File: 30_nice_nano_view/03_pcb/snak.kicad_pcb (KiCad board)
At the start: 2 copper layers, 114 x 99 mm, 162 parts

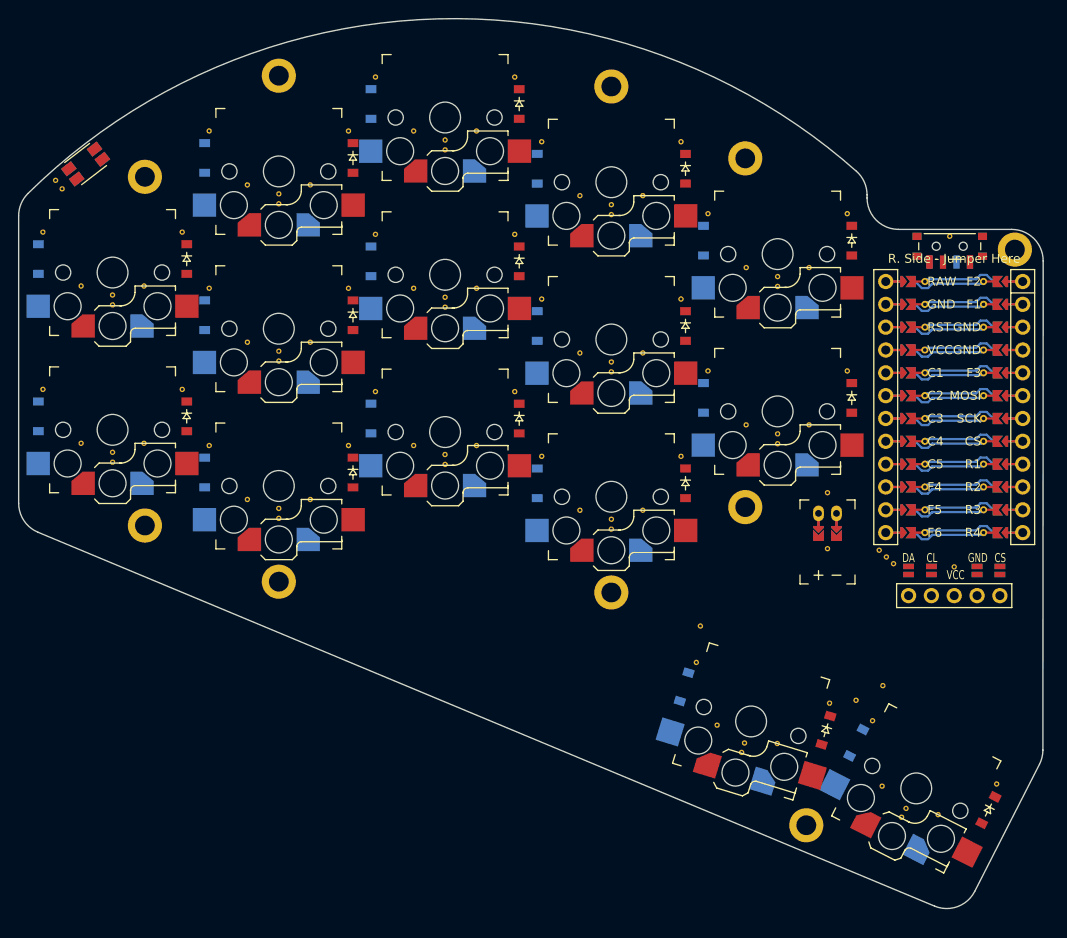
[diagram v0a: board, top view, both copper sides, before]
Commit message: update
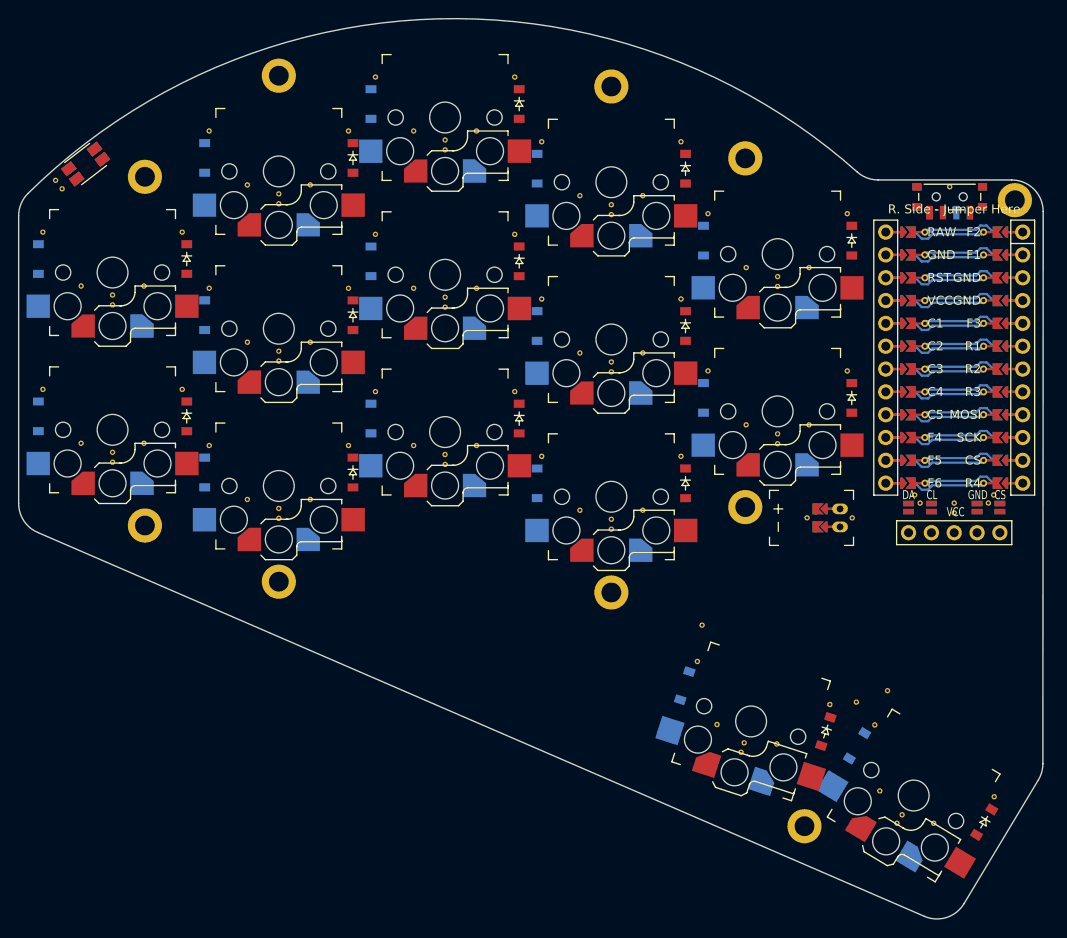
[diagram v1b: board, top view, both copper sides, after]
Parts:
- removed the REF** at (179.6, 89.5)
- removed the REF** at (179.8, 112.9)
- removed the REF** at (198.4, 121.9)
- removed the REF** at (174.0, 117.4)
- removed the REF** at (191.9, 125.3)
- removed the REF** at (165.0, 108.4)
- removed the REF** at (184.6, 114.9)
- removed the REF** at (167.3, 115.4)
- removed the REF** at (185.6, 122.1)
- removed the REF** at (170.0, 118.4)
- removed the REF** at (187.8, 125.6)
- removed the REF** at (170.3, 117.3)
- removed the REF** at (188.3, 124.6)
- removed the REF** at (182.7, 112.6)
- removed the REF** at (165.4, 104.3)
- removed the REF** at (185.7, 111.0)
- removed the REF** at (186.9, 97.4)
- removed the REF** at (186.1, 96.7)
- removed the REF** at (185.3, 95.9)
- removed the REF** at (193.7, 97.8)
- removed the REF** at (193.2, 61.0)
- removed the REF** at (179.6, 95.7)
- added REF**: VIA-0.6mm, VIA-0.6mm, F.Cu at (193.2, 55.5)
- added REF**: VIA-0.6mm, VIA-0.6mm, F.Cu at (177.3, 92.3)
- added REF**: VIA-0.6mm, VIA-0.6mm, F.Cu at (182.3, 92.3)
- added REF**: VIA-0.6mm, VIA-0.6mm, F.Cu at (179.8, 113.1)
- added REF**: VIA-0.6mm, VIA-0.6mm, F.Cu at (198.1, 123.3)
- added REF**: VIA-0.6mm, VIA-0.6mm, F.Cu at (173.9, 117.5)
- added REF**: VIA-0.6mm, VIA-0.6mm, F.Cu at (191.4, 126.3)
- added REF**: VIA-0.6mm, VIA-0.6mm, F.Cu at (165.1, 108.3)
- added REF**: VIA-0.6mm, VIA-0.6mm, F.Cu at (184.8, 115.3)
- added REF**: VIA-0.6mm, VIA-0.6mm, F.Cu at (167.3, 115.3)
- added REF**: VIA-0.6mm, VIA-0.6mm, F.Cu at (185.4, 122.7)
- added REF**: VIA-0.6mm, VIA-0.6mm, F.Cu at (169.9, 118.4)
- added REF**: VIA-0.6mm, VIA-0.6mm, F.Cu at (187.3, 126.3)
- added REF**: VIA-0.6mm, VIA-0.6mm, F.Cu at (170.3, 117.3)
- added REF**: VIA-0.6mm, VIA-0.6mm, F.Cu at (187.9, 125.3)
- added REF**: VIA-0.6mm, VIA-0.6mm, F.Cu at (182.8, 112.8)
- added REF**: VIA-0.6mm, VIA-0.6mm, F.Cu at (165.6, 104.2)
- added REF**: VIA-0.6mm, VIA-0.6mm, F.Cu at (186.2, 111.5)
- added REF**: VIA-0.6mm, VIA-0.6mm, F.Cu at (189.2, 89.8)
- added REF**: VIA-0.6mm, VIA-0.6mm, F.Cu at (198.1, 89.8)
- added REF**: VIA-0.6mm, VIA-0.6mm, F.Cu at (193.7, 90.7)
- added REF**: VIA-0.6mm, VIA-0.6mm, F.Cu at (189.8, 90.7)
- added REF**: VIA-0.6mm, VIA-0.6mm, F.Cu at (197.5, 90.7)
- added REF**: VIA-0.6mm, VIA-0.6mm, F.Cu at (193.7, 91.8)
- moved DISP1 7.00 mm to (193.7, 77.2)
- moved H10 5.50 mm to (200.4, 57.0)
- moved MCU1 5.50 mm to (193.7, 73.2)
- moved SW1 5.50 mm to (193.2, 56.6)
- moved JST1 1.49 mm to (180.9, 92.3), turned to 270 degrees
- moved D15 1.43 mm to (197.0, 126.2), turned to 239 degrees
- moved S15 0.85 mm to (189.1, 123.2), turned to 149 degrees
- moved D30 0.35 mm to (182.8, 117.7), turned to 239 degrees
- moved H9 0.23 mm to (177.0, 126.6), turned to -18 degrees
- moved D29 0.15 mm to (163.7, 111.0), turned to 252 degrees
- moved D14 0.15 mm to (179.4, 116.1), turned to 252 degrees
- turned S14 to 162 degrees
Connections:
- MCU1 pad 114: R3 -> CS
- MCU1 pad 115: R2 -> SCK
- MCU1 pad 116: R1 -> MOSI
- MCU1 pad 117: CS -> R3
- MCU1 pad 118: SCK -> R2
- MCU1 pad 119: MOSI -> R1
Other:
- board size 114 x 99 mm -> 114 x 100.2 mm
